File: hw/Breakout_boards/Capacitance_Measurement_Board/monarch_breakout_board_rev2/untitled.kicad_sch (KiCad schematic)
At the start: 12 parts, among them J1 2200980471, J2 2200980471, J3 2200980471, J4 2200980471

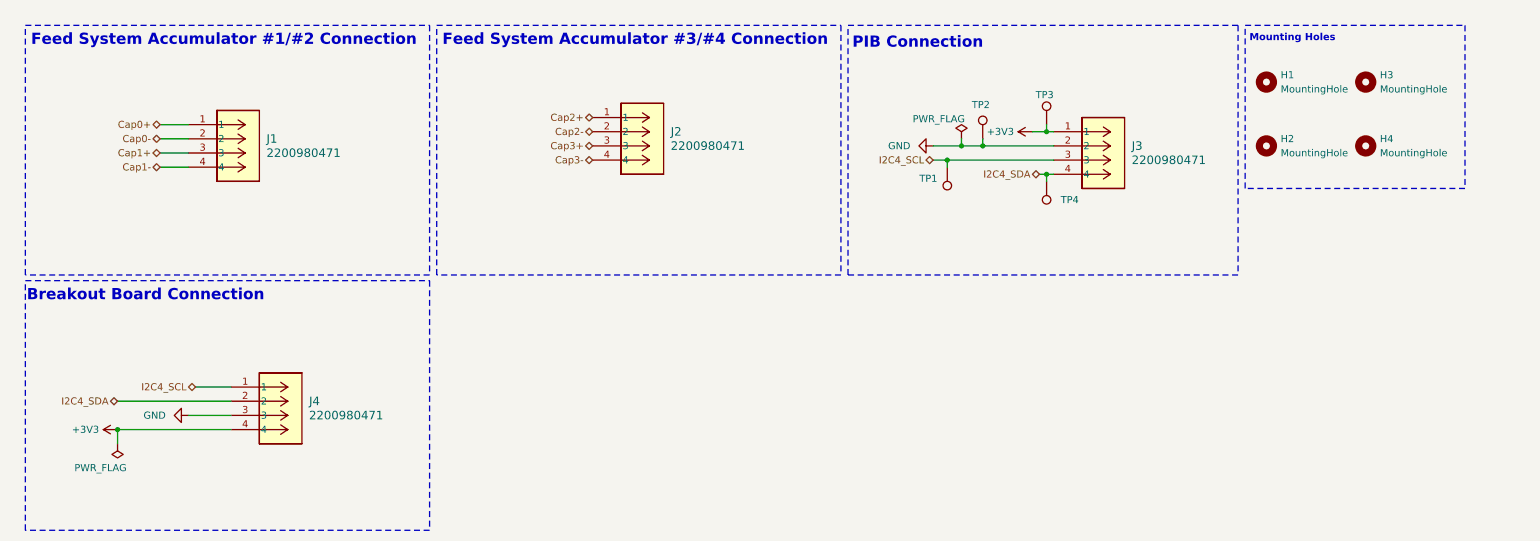
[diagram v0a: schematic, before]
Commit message: New REV2 Breakout Board Schematic Done
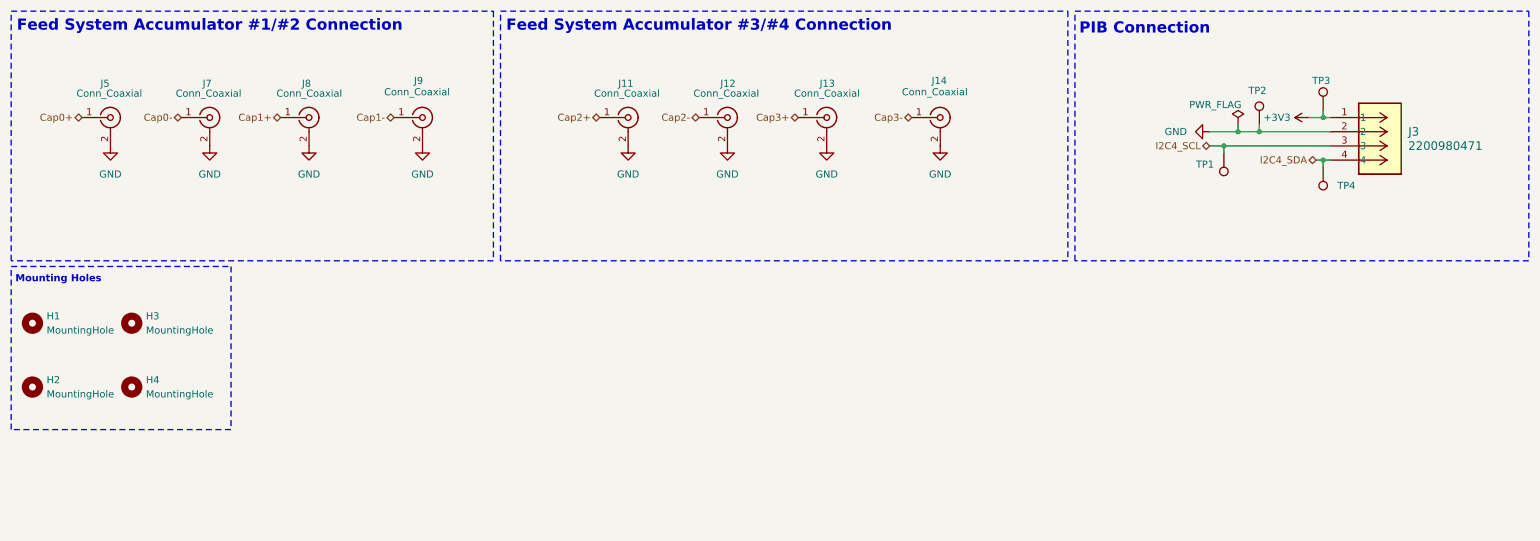
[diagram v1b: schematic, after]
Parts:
- removed J1, J2, J4: 2200980471, Connector_Molex_Micro-Lock-Plus:Molex_Micro-Lock_2200980471_1x04_P1.25mm_Horizontal, symbol 5037630491:5037630491
- added J11, J12, J13, J14, J5, J7, J8, J9: Conn_Coaxial, symbol Connector:Conn_Coaxial
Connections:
- net Cap0+: now also J5.1 (In)
- net Cap0-: now also J7.1 (In)
- net Cap1+: now also J8.1 (In)
- net Cap1-: now also J9.1 (In)
- net Cap2+: now also J11.1 (In)
- net Cap2-: now also J12.1 (In)
- net Cap3+: now also J13.1 (In)
- net Cap3-: now also J14.1 (In)
- net GND: now also J11.2 (Ext), J12.2 (Ext), J13.2 (Ext), J14.2 (Ext), J5.2 (Ext), J7.2 (Ext), J8.2 (Ext), J9.2 (Ext)
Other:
- note removed: "Breakout Board Connection"
- company: (none) -> EP + LASSI LAB
- title: (none) -> Breakout Board
- moved on the sheet: H1, H2, H3, H4, J3, TP1, TP2, TP3, TP4
